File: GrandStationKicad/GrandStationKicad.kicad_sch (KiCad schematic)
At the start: 19 parts, among them J1 Conn_01x04_Female, J2 Conn_01x06_Female, U1 STM32F030F4Px, U2 Ai-Thinker-Ra-02, Y1 16MHz

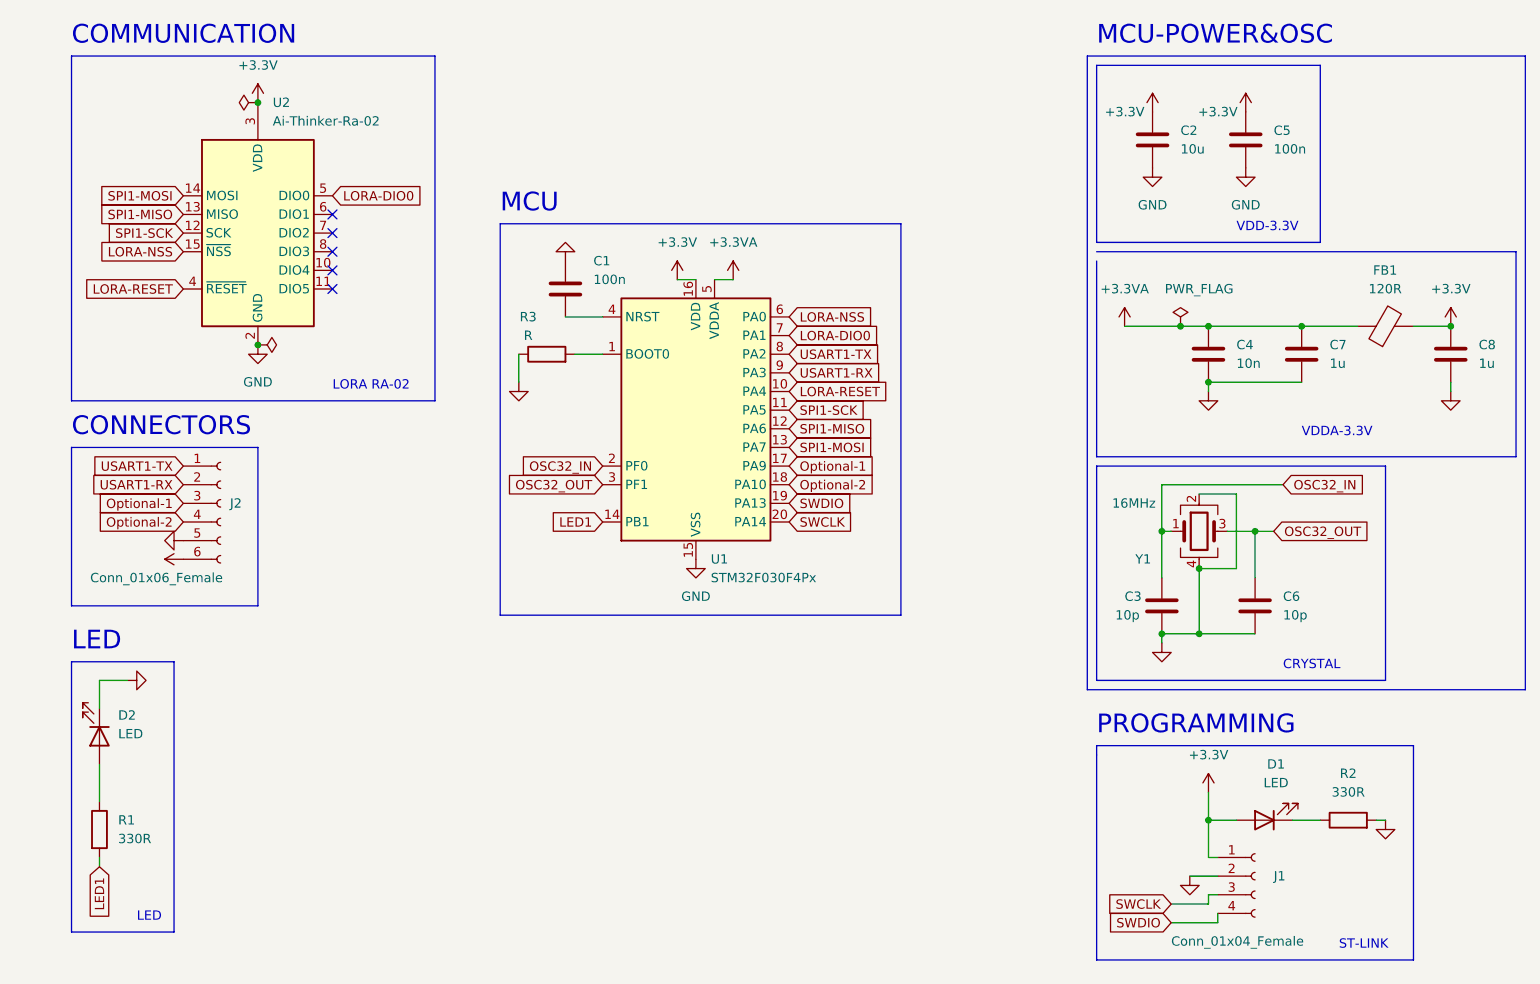
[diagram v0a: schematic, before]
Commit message: update4-12-23
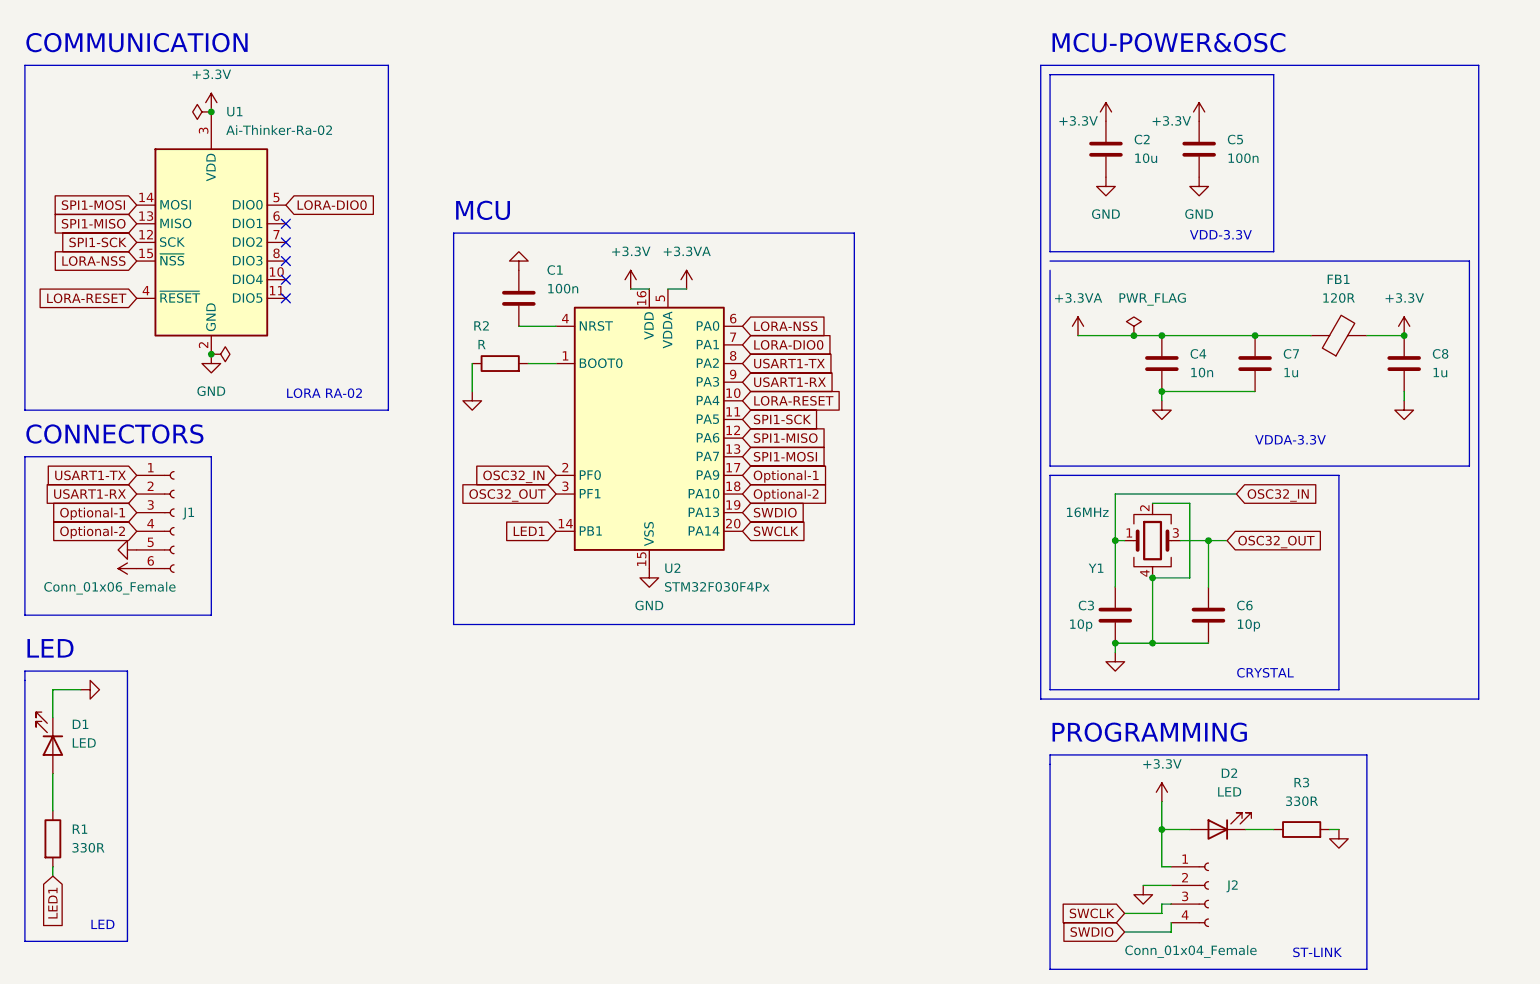
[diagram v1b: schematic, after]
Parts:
- removed J1: Conn_01x04_Female, Connector_PinSocket_2.54mm:PinSocket_1x04_P2.54mm_Vertical, symbol Connector:Conn_01x04_Female
- removed J2: Conn_01x06_Female, Connector_PinSocket_2.54mm:PinSocket_1x06_P2.54mm_Vertical, symbol Connector:Conn_01x06_Female
- removed U1: STM32F030F4Px, Package_SO:TSSOP-20_4.4x6.5mm_P0.65mm, symbol MCU_ST_STM32F0:STM32F030F4Px
- removed U2: Ai-Thinker-Ra-02, RF_Module:Ai-Thinker-Ra-01-LoRa, symbol RF_Module:Ai-Thinker-Ra-02
- added J1: Conn_01x06_Female, Connector_PinSocket_2.54mm:PinSocket_1x06_P2.54mm_Vertical, symbol Connector:Conn_01x06_Female
- added J2: Conn_01x04_Female, Connector_PinSocket_2.54mm:PinSocket_1x04_P2.54mm_Vertical, symbol Connector:Conn_01x04_Female
- added U1: Ai-Thinker-Ra-02, RF_Module:Ai-Thinker-Ra-01-LoRa, symbol RF_Module:Ai-Thinker-Ra-02
- added U2: STM32F030F4Px, Package_SO:TSSOP-20_4.4x6.5mm_P0.65mm, symbol MCU_ST_STM32F0:STM32F030F4Px
- R2: value 330R -> R
- R3: value R -> 330R
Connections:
- net +3.3V: now also D2.2 (A), J1.6 (Pin_6), J2.1 (Pin_1), U1.3 (VDD), U2.16 (VDD); no longer D1.2 (A)
- net +3.3VA: now also U2.5 (VDDA)
- net GND: now also D1.1 (K), R2.1, R3.2, J1.5 (Pin_5), J2.2 (Pin_2), U1.1 (GND), U1.16 (GND), U1.2 (GND), U1.9 (GND), U2.15 (VSS); no longer D2.1 (K), R2.2, R3.1
- net LED1: now also U2.14 (PB1)
- net LORA-DIO0: now also U1.5 (DIO0), U2.7 (PA1)
- net LORA-NSS: now also U1.15 (~{NSS}), U2.6 (PA0)
- net LORA-RESET: now also U1.4 (~{RESET}), U2.10 (PA4)
- net OSC32_IN: now also U2.2 (PF0)
- net OSC32_OUT: now also U2.3 (PF1)
- net Optional-1: now also J1.3 (Pin_3), U2.17 (PA9)
- net Optional-2: now also J1.4 (Pin_4), U2.18 (PA10)
- net SPI1-MISO: now also U1.13 (MISO), U2.12 (PA6)
- net SPI1-MOSI: now also U1.14 (MOSI), U2.13 (PA7)
- net SPI1-SCK: now also U1.12 (SCK), U2.11 (PA5)
- net SWCLK: now also J2.3 (Pin_3), U2.20 (PA14)
- net SWDIO: now also J2.4 (Pin_4), U2.19 (PA13)
- net USART1-RX: now also J1.2 (Pin_2), U2.9 (PA3)
- net USART1-TX: now also J1.1 (Pin_1), U2.8 (PA2)
- net at C1.2: now also U2.4 (NRST)
- net at R1.1: now also D1.2 (A); no longer D2.2 (A)
- new net: D2.1 (K), R3.1
- new net: R2.2, U2.1 (BOOT0)
